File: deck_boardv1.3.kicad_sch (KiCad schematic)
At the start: 29 parts, among them J1 430450800, U1 Raspberry Pi Zero 2 W, U2 LT8610AC, U3 DIGI XBee-PRO 900HP RF Module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, U4 ADP7159

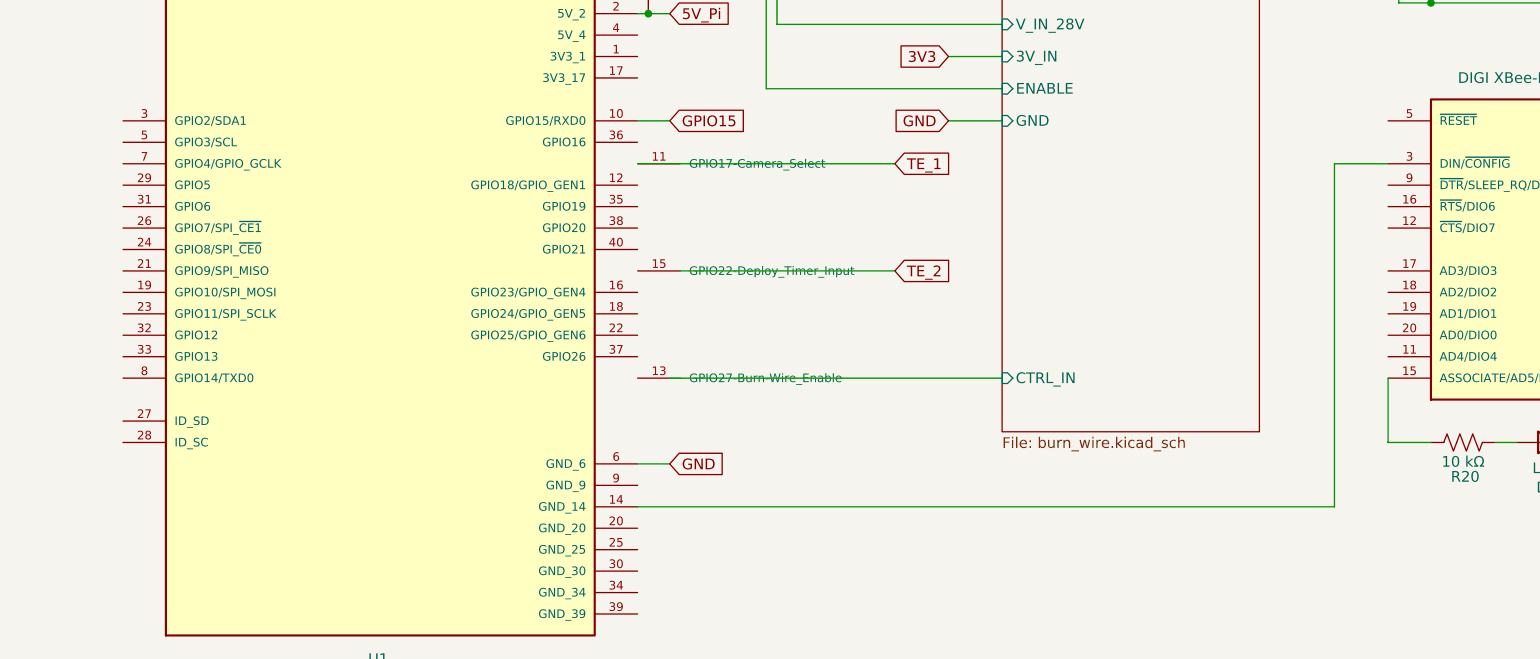
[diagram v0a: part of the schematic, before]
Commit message: Finished PCB, ready to print
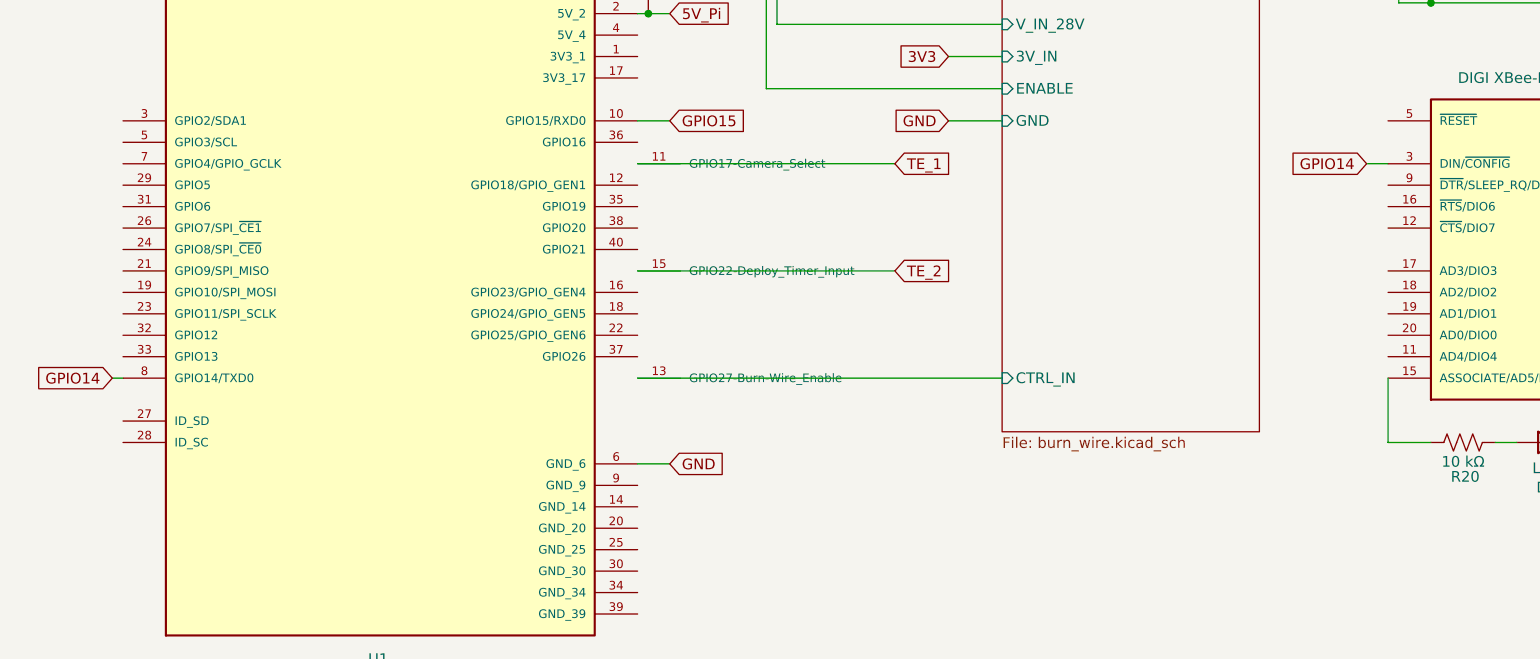
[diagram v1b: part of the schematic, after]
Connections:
- net Burn-Wire Circuit/CTRL_IN: now also U1.13 (GPIO27-Burn-Wire_Enable)
- net TE_2: now also U1.15 (GPIO22-Deploy_Timer_Input)
- net at U1.14 (GND_14): no longer U3.3 (DIN/~{CONFIG})
- net GPIO14: now reaches U1.8 (GPIO14/TXD0)
- net GPIO14: now also U3.3 (DIN/~{CONFIG})
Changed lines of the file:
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@@
 	(wire
 		(pts
-			(xy 173.99 120.65) (xy 167.64 120.65)
+			(xy 171.45 120.65) (xy 173.99 120.65)
 		)
 		(stroke
@@
 	(wire
 		(pts
+			(xy 85.09 133.35) (xy 115.57 133.35)
+		)
+		(stroke
+			(width 0)
+			(type default)
+		)
+	)
+	(wire
+		(pts
 			(xy 80.01 50.8) (xy 82.55 50.8)
 		)
@@
 	(wire
 		(pts
-			(xy 167.64 120.65) (xy 167.64 161.29)
-		)
-		(stroke
-			(width 0)
-			(type default)
-		)
-	)
-	(wire
-		(pts
-			(xy 85.09 161.29) (xy 167.64 161.29)
-		)
-		(stroke
-			(width 0)
-			(type default)
-		)
-	)
-	(wire
-		(pts
 			(xy 232.41 115.57) (xy 242.57 115.57)
 		)
@@
 	(wire
 		(pts
-			(xy 121.92 107.95) (xy 128.27 107.95)
+			(xy 22.86 146.05) (xy 24.13 146.05)
 		)
 		(stroke
@@
 	(wire
 		(pts
-			(xy 129.54 58.42) (xy 135.89 58.42)
+			(xy 121.92 107.95) (xy 128.27 107.95)
 		)
 		(stroke
@@
 	(wire
 		(pts
-			(xy 139.7 66.04) (xy 139.7 63.5)
+			(xy 129.54 58.42) (xy 135.89 58.42)
 		)
 		(stroke
@@
 	(wire
 		(pts
-			(xy 80.01 39.37) (xy 85.09 39.37)
+			(xy 139.7 66.04) (xy 139.7 63.5)
 		)
 		(stroke
@@
 	(wire
 		(pts
-			(xy 229.87 76.2) (xy 242.57 76.2)
+			(xy 80.01 39.37) (xy 85.09 39.37)
 		)
 		(stroke
@@
 	(wire
 		(pts
-			(xy 41.91 27.94) (xy 52.07 27.94)
+			(xy 229.87 76.2) (xy 242.57 76.2)
 		)
 		(stroke
@@
 	(wire
 		(pts
-			(xy 226.06 115.57) (xy 232.41 115.57)
+			(xy 41.91 27.94) (xy 52.07 27.94)
 		)
 		(stroke
@@
 	(wire
 		(pts
-			(xy 90.17 133.35) (xy 115.57 133.35)
+			(xy 226.06 115.57) (xy 232.41 115.57)
 		)
 		(stroke
@@
 	(wire
 		(pts
+			(xy 85.09 146.05) (xy 128.27 146.05)
+		)
+		(stroke
+			(width 0)
+			(type default)
+		)
+	)
+	(wire
+		(pts
 			(xy 139.7 63.5) (xy 139.7 49.53)
 		)
@@
 	(wire
 		(pts
-			(xy 88.9 146.05) (xy 128.27 146.05)
-		)
-		(stroke
-			(width 0)
-			(type default)
-		)
-	)
-	(wire
-		(pts
 			(xy 86.36 102.87) (xy 88.9 102.87)
 		)
@@
 		)
 	)
+	(global_label "GPIO14"
+		(shape input)
+		(at 22.86 146.05 180)
+		(fields_autoplaced yes)
+		(effects
+			(font
+				(size 1.27 1.27)
+			)
+			(justify right)
+		)
+		(property "Intersheetrefs" "${INTERSHEET_REFS}"
+			(at 12.9805 146.05 0)
+			(effects
+				(font
+					(size 1.27 1.27)
+				)
+				(justify right)
+				(hide yes)
+			)
+		)
+	)
 	(global_label "3V3"
 		(shape input)
@@
 		)
 	)
+	(global_label "GPIO14"
+		(shape input)
+		(at 171.45 120.65 180)
+		(fields_autoplaced yes)
+		(effects
+			(font
+				(size 1.27 1.27)
+			)
+			(justify right)
+		)
+		(property "Intersheetrefs" "${INTERSHEET_REFS}"
+			(at 161.5705 120.65 0)
+			(effects
+				(font
+					(size 1.27 1.27)
+				)
+				(justify right)
+				(hide yes)
+			)
+		)
+	)
 	(global_label "TE_1"
 		(shape input)
@@
 		)
 		(instances
-			(project "deck_boardv1.1"
+			(project "deck_boardv1.2"
 				(path "/0dd6c749-d328-44a2-b3d4-206fc5899db9"
 					(page "3")
@@
 		)
 		(instances
-			(project "deck_boardv1.1"
+			(project "deck_boardv1.2"
 				(path "/0dd6c749-d328-44a2-b3d4-206fc5899db9"
 					(page "2")
@@
 		)
 		(instances
-			(project "deck_boardv1.1"
+			(project "deck_boardv1.2"
 				(path "/0dd6c749-d328-44a2-b3d4-206fc5899db9"
 					(page "4")
